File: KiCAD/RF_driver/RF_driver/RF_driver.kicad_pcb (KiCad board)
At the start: 2 copper layers, 46.8 x 46 mm, 18 parts, among them J1 Conn_Coaxial, J2 Conn_01x02_Pin, U1 TLV3542IDR

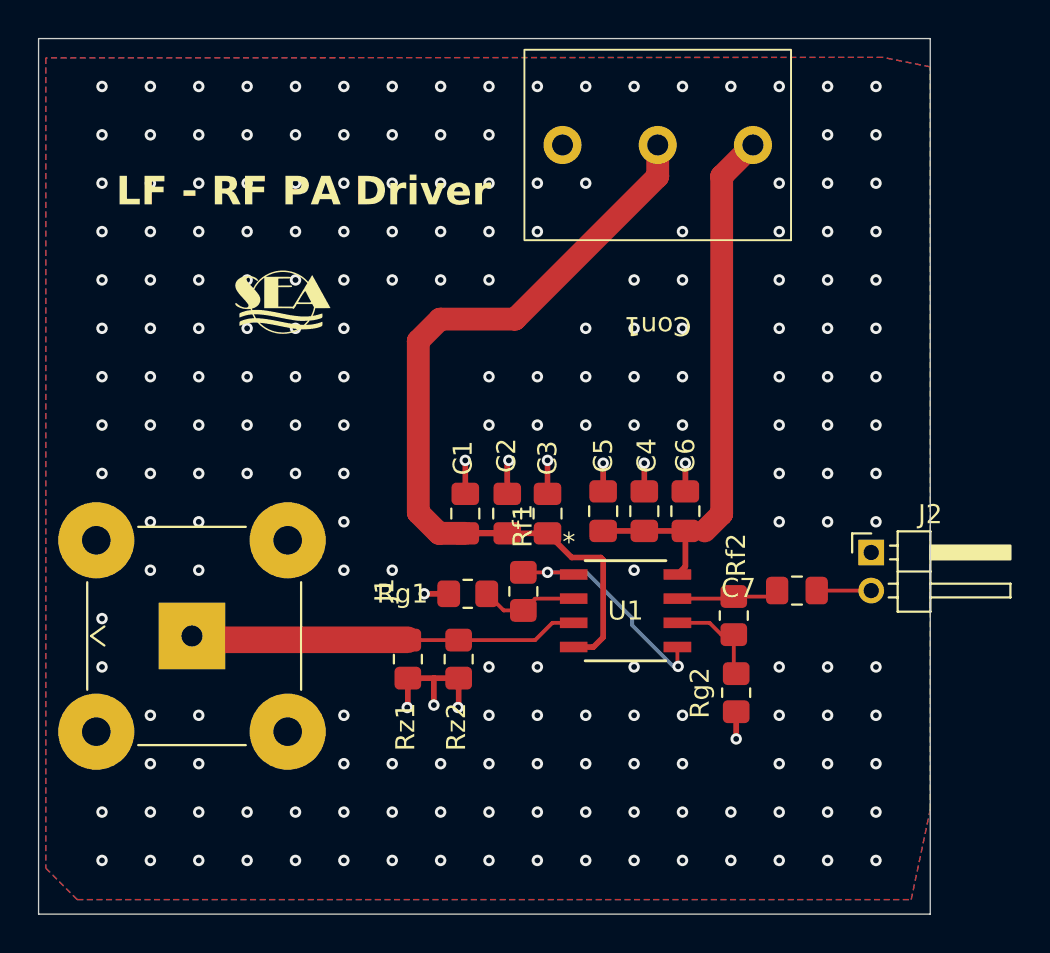
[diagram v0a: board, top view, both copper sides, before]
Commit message: Design ordered
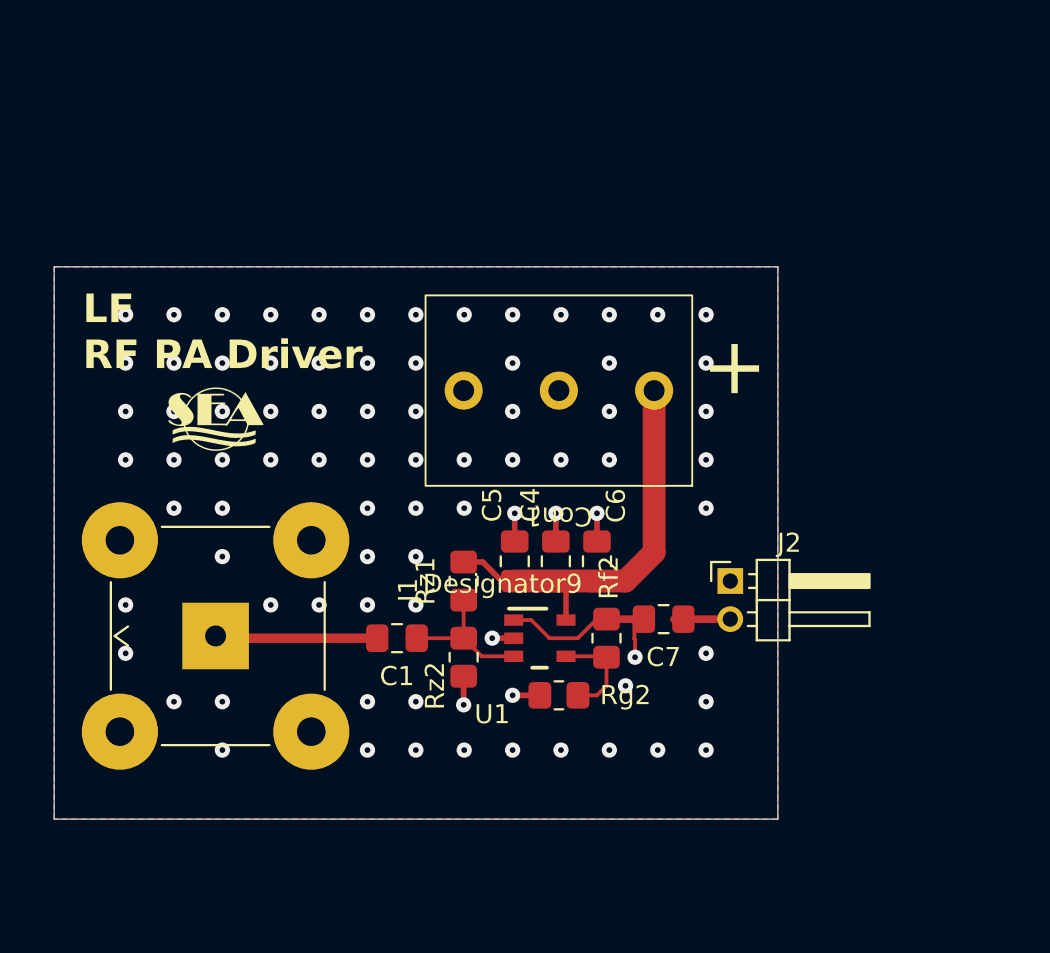
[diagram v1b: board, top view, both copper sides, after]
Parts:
- removed C2: 10nF, Capacitor_SMD:C_0805_2012Metric_Pad1.18x1.45mm_HandSolder
- removed C3: 1nF, Capacitor_SMD:C_0805_2012Metric_Pad1.18x1.45mm_HandSolder
- removed Rf1, Rg1: 10k, Resistor_SMD:R_0805_2012Metric_Pad1.20x1.40mm_HandSolder
- C7: value 1nF -> 100nF
- Rf2: value 10k -> 0
- U1: value TLV3542IDR -> TLV3541IDBVR; footprint RF_PA:D8_TEX -> RF_PA:DBV0005A_N
- moved Con1 13.9 mm to (126.0, 84.0)
- moved Rg2 9.31 mm to (126.0, 91.0), turned to 0 degrees
- moved J2 7.55 mm to (135.0, 85.0)
- moved C1 7.46 mm to (117.5, 88.0), turned to 180 degrees
- moved C7 7.16 mm to (131.5, 87.0)
- moved G*** 7.07 mm to (108.0, 76.5)
- moved Rf2 6.79 mm to (128.5, 88.0)
- moved C4 5.34 mm to (125.8, 84.0)
- moved C6 5.34 mm to (128.0, 84.0)
- moved C5 5.34 mm to (123.7, 84.0)
- moved Rz1 5.04 mm to (121.0, 85.0)
- moved U1 4.73 mm to (125.0, 88.0)
- moved J1 1.24 mm to (108.0, 87.9)
- moved Rz2 0.28 mm to (121.0, 89.0)
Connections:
- C1 pad 1: -12V -> Net-(U1-IN+)
- C1 pad 2: GND -> Net-(J1-In)
- C4 pad 1: +12V -> +5V
- C5 pad 1: +12V -> +5V
- C6 pad 1: +12V -> +5V
- C7 pad 2: Net-(U1-OUT_B) -> Net-(U1-OUT)
- Con1 pad 1: +12V -> +5V
- Con1 pad 2: -12V -> GND
- Rf2 pad 1: Net-(U1--IN_B) -> Net-(U1-IN-)
- Rf2 pad 2: Net-(U1-OUT_B) -> Net-(U1-OUT)
- Rg2 pad 2: Net-(U1--IN_B) -> Net-(U1-IN-)
- Rz1 pad 1: GND -> Net-(U1-IN+)
- Rz1 pad 2: Net-(J1-In) -> +5V
- Rz2 pad 2: Net-(J1-In) -> Net-(U1-IN+)
- U1 pad 1: Net-(U1-+IN_B) -> Net-(U1-OUT)
- U1 pad 2: Net-(U1-IN_A) -> GND
- U1 pad 3: Net-(J1-In) -> Net-(U1-IN+)
- U1 pad 4: -12V -> Net-(U1-IN-)
- U1 pad 5: Net-(U1-+IN_B) -> +5V
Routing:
- net -12V: track 45.6 -> 0.00 mm
- net +12V: track 29.1 -> 0.00 mm
- net +5V: track 0.00 -> 26.1 mm
- net Net-(U1-+IN_B): track 12.9 -> 0.00 mm, vias 2 -> 0
- net GND: track 19.6 -> 8.50 mm, vias 207 -> 82
- net Net-(J1-In): track 20.4 -> 9.28 mm
- net Net-(U1-OUT): track 0.00 -> 9.16 mm, vias 0 -> 1
- net Net-(U1-IN+): track 0.00 -> 7.98 mm
- net Net-(U1-OUT_B): track 5.42 -> 0.00 mm
- net Net-(U1--IN_B): track 5.32 -> 0.00 mm
- net Net-(U1-IN_A): track 5.18 -> 0.00 mm
- net Net-(U1-IN-): track 0.00 -> 4.85 mm
- net Net-(J2-Pin_2): track 2.86 -> 2.36 mm
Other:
- board size 46.8 x 46 mm -> 38 x 29 mm
- board text added: "+"
- board text added: "LF RF PA Driver"
- board text removed: "LF - RF PA Driver"
